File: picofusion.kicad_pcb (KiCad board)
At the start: 4 copper layers, 25.5 x 25.5 mm, 69 parts, among them J1 NORTH, J2 EAST, J3 WEST, J4 SOUTH, U1 W25Q16, U2 RP2040, U3 TLV71333PDQN, U4 ICM-20602, U5 MMC5983MA, U6 ICP20100, U7 TJA1051TK-3, Y1 12MHz

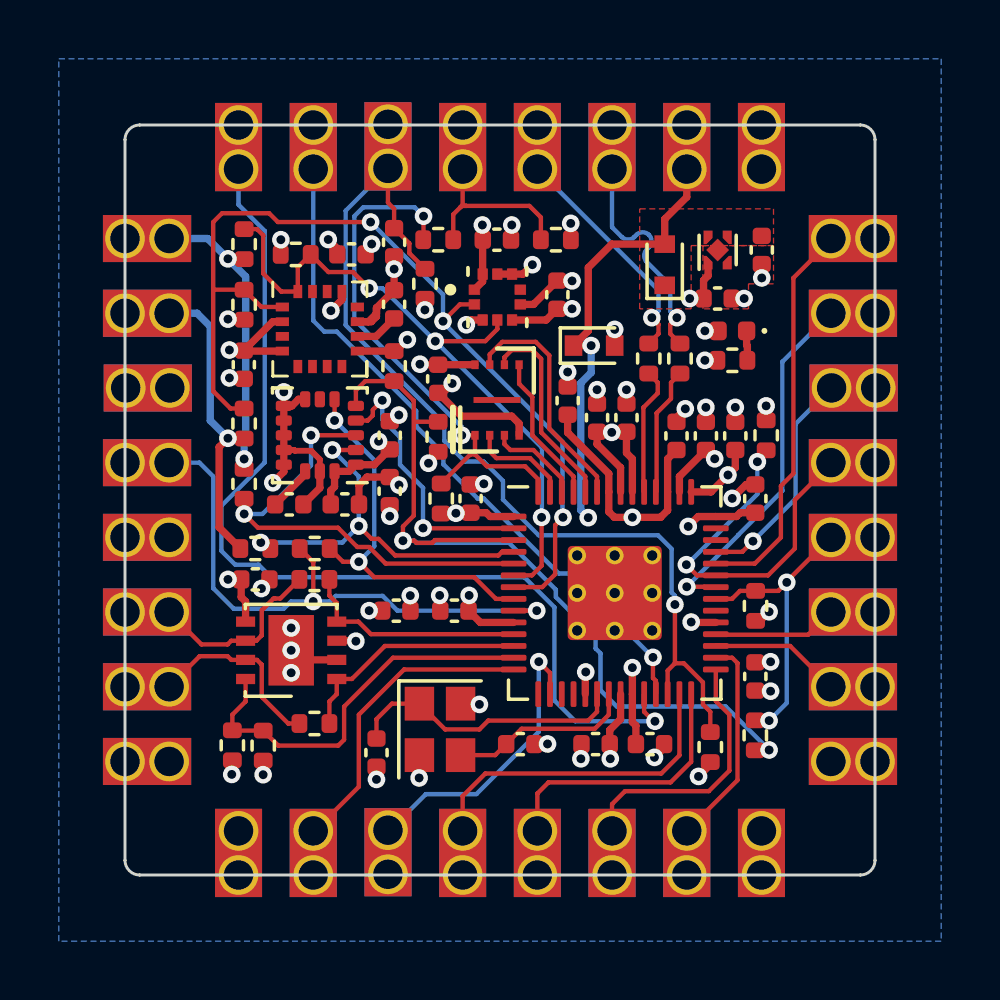
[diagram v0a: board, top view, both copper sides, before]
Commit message: R02B: more work
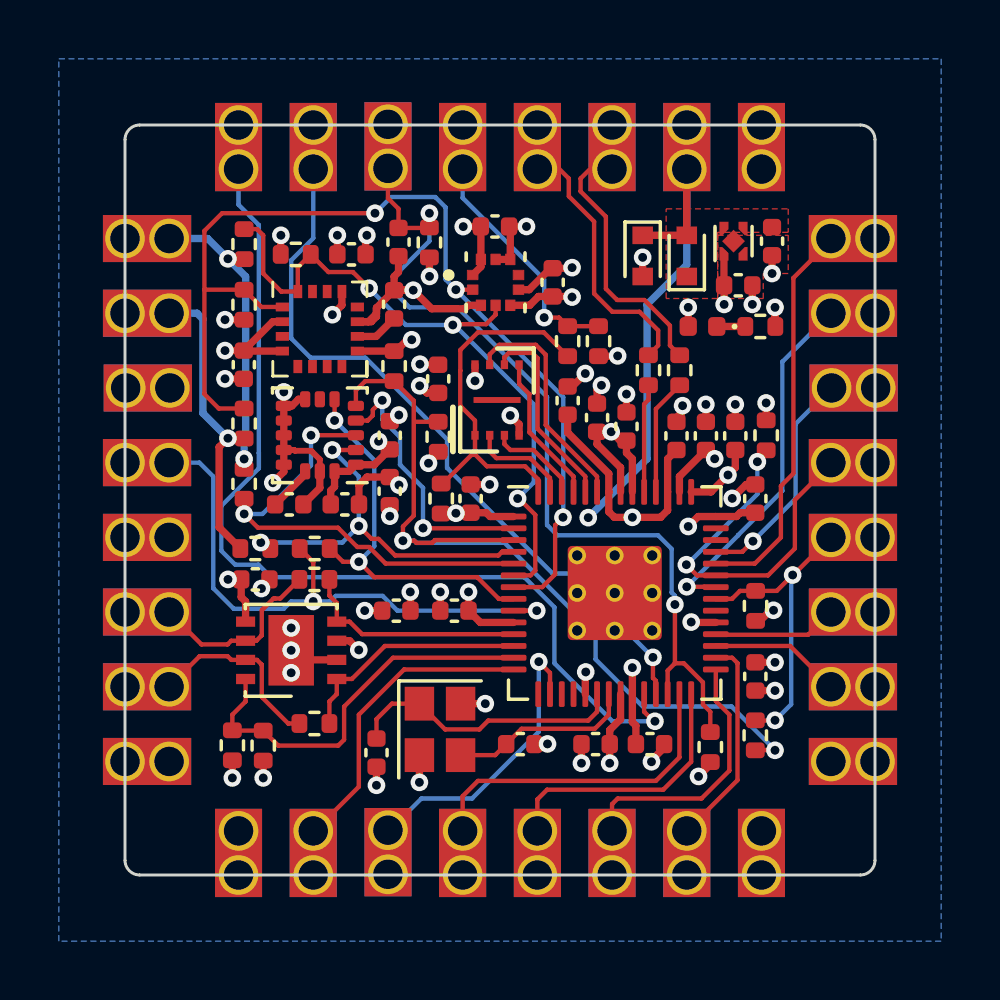
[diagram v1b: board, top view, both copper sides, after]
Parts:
- moved R20 5.59 mm to (162.3, 34.6), turned to -90 degrees
- moved R19 3.74 mm to (163.3, 34.6), turned to -90 degrees
- moved D1 3.47 mm to (164.8, 31.7), turned to -90 degrees
- moved R6 1.49 mm to (168.8, 34.1), turned to 0 degrees
- moved R1 1.42 mm to (157.6, 31.2)
- moved D2 1.03 mm to (166.9, 34.1)
- moved C16 0.83 mm to (168.1, 32.7)
- moved D3 0.81 mm to (166.3, 31.7)
- moved U3 0.62 mm to (167.9, 31.2)
- moved U6 0.50 mm to (159.8, 32.6)
- moved C14 0.46 mm to (169.2, 31.2)
- moved C23 0.45 mm to (159.8, 30.7)
- moved C22 0.45 mm to (161.8, 32.6)
- moved R2 0.40 mm to (165.0, 35.6)
- moved R3 0.40 mm to (166.1, 35.6)
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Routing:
- net /QSPI_nCS: track 17.9 -> 12.4 mm, vias 2 -> 0
- net GND: track 40.4 -> 45.3 mm, vias 43 -> 42
- net /RUN: track 32.9 -> 30.6 mm, vias 1 -> 2
- net /I2C0_SCL: track 32.9 -> 35.2 mm
- net +5V: track 34.5 -> 36.8 mm, vias 4 -> 3
- net /BOOTSEL: track 6.35 -> 8.17 mm, vias 0 -> 1
- net /USB_DN: track 7.91 -> 9.46 mm, vias 1 -> 0
- net /USB_DP: track 7.96 -> 9.46 mm, vias 1 -> 0
- net /SWDIO: track 24.3 -> 25.8 mm
- net /SWCLK: track 34.1 -> 33.1 mm
- net +3V3: track 43.1 -> 43.8 mm, vias 26 -> 27
- net /USB_MCU_DP: track 4.33 -> 3.69 mm
